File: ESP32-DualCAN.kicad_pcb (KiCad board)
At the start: 2 copper layers, 19.6 x 38.8 mm, 28 parts, among them J1 Molex 70553 6p, J2 Conn_01x10_Socket, J3 Conn_01x10_Socket, J4 holes, J5 pads, J6 holes, J7 pads, U1 LV2862Y, U2 ESP32-C6-SuperMini, U3 TCAN1044AV, U4 TCAN1044AV

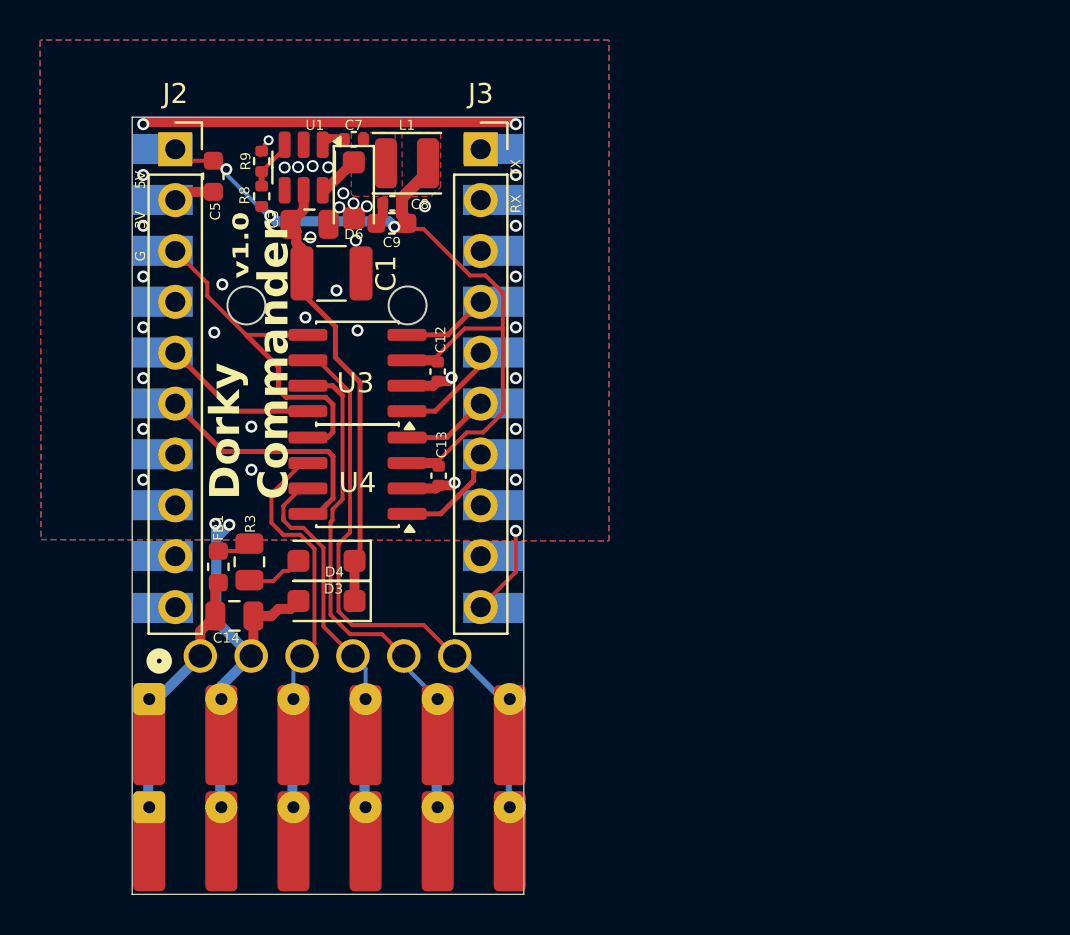
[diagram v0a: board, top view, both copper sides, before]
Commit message: horizontal layout
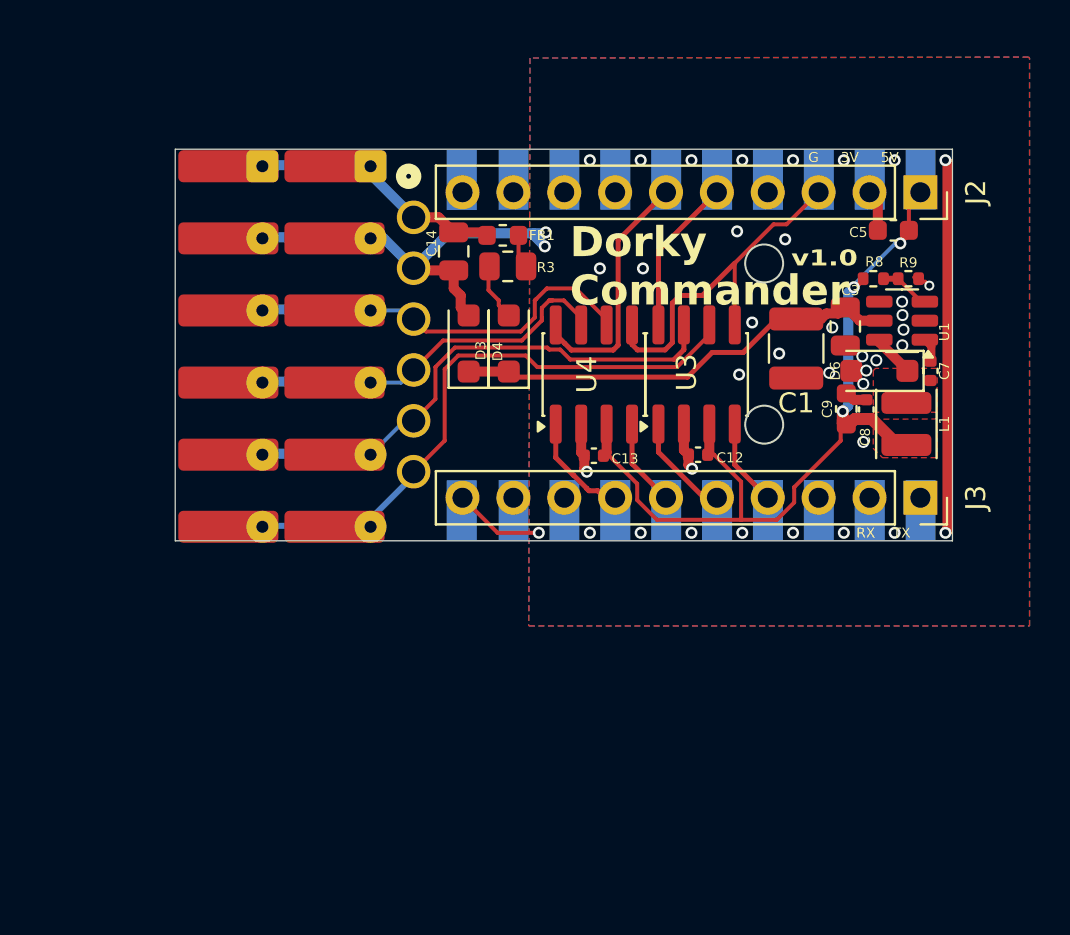
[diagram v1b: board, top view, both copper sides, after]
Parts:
- moved J2 37.3 mm to (158.8, 83.0), turned to -90 degrees
- moved C5 34.1 mm to (157.5, 84.9), turned to 180 degrees
- moved J7 33.9 mm to (124.3, 81.7), turned to -90 degrees
- moved R9 32.8 mm to (158.2, 87.3), turned to 180 degrees
- moved J4 32.5 mm to (126.0, 81.7), turned to -90 degrees
- moved C7 31.0 mm to (159.3, 91.9), turned to -90 degrees
- moved U1 30.8 mm to (157.9, 89.4), turned to 180 degrees
- moved R8 30.8 mm to (156.5, 87.3), turned to 180 degrees
- moved J5 29.9 mm to (129.6, 81.7), turned to -90 degrees
- moved J6 28.8 mm to (131.4, 81.7), turned to -90 degrees
- moved L1 28.1 mm to (158.2, 94.6), turned to -90 degrees
- moved J3 28.0 mm to (158.8, 98.2), turned to -90 degrees
- moved D6 27.7 mm to (156.8, 91.9), turned to 180 degrees
- moved C3 27.2 mm to (155.1, 89.7), turned to -90 degrees
- moved C8 25.8 mm to (156.2, 93.8), turned to 90 degrees
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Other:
- board size 19.6 x 38.8 mm -> 38.8 x 19.6 mm
